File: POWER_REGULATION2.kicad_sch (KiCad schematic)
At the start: 73 parts, among them Q8 FDV301N, U19 NL17SZ17XV5T2G, U21 NC7WZ07P6X, U22 TPS65400RGZT, U40 TPS22918DBVR, U9 SIP32510DT-T1-GE3

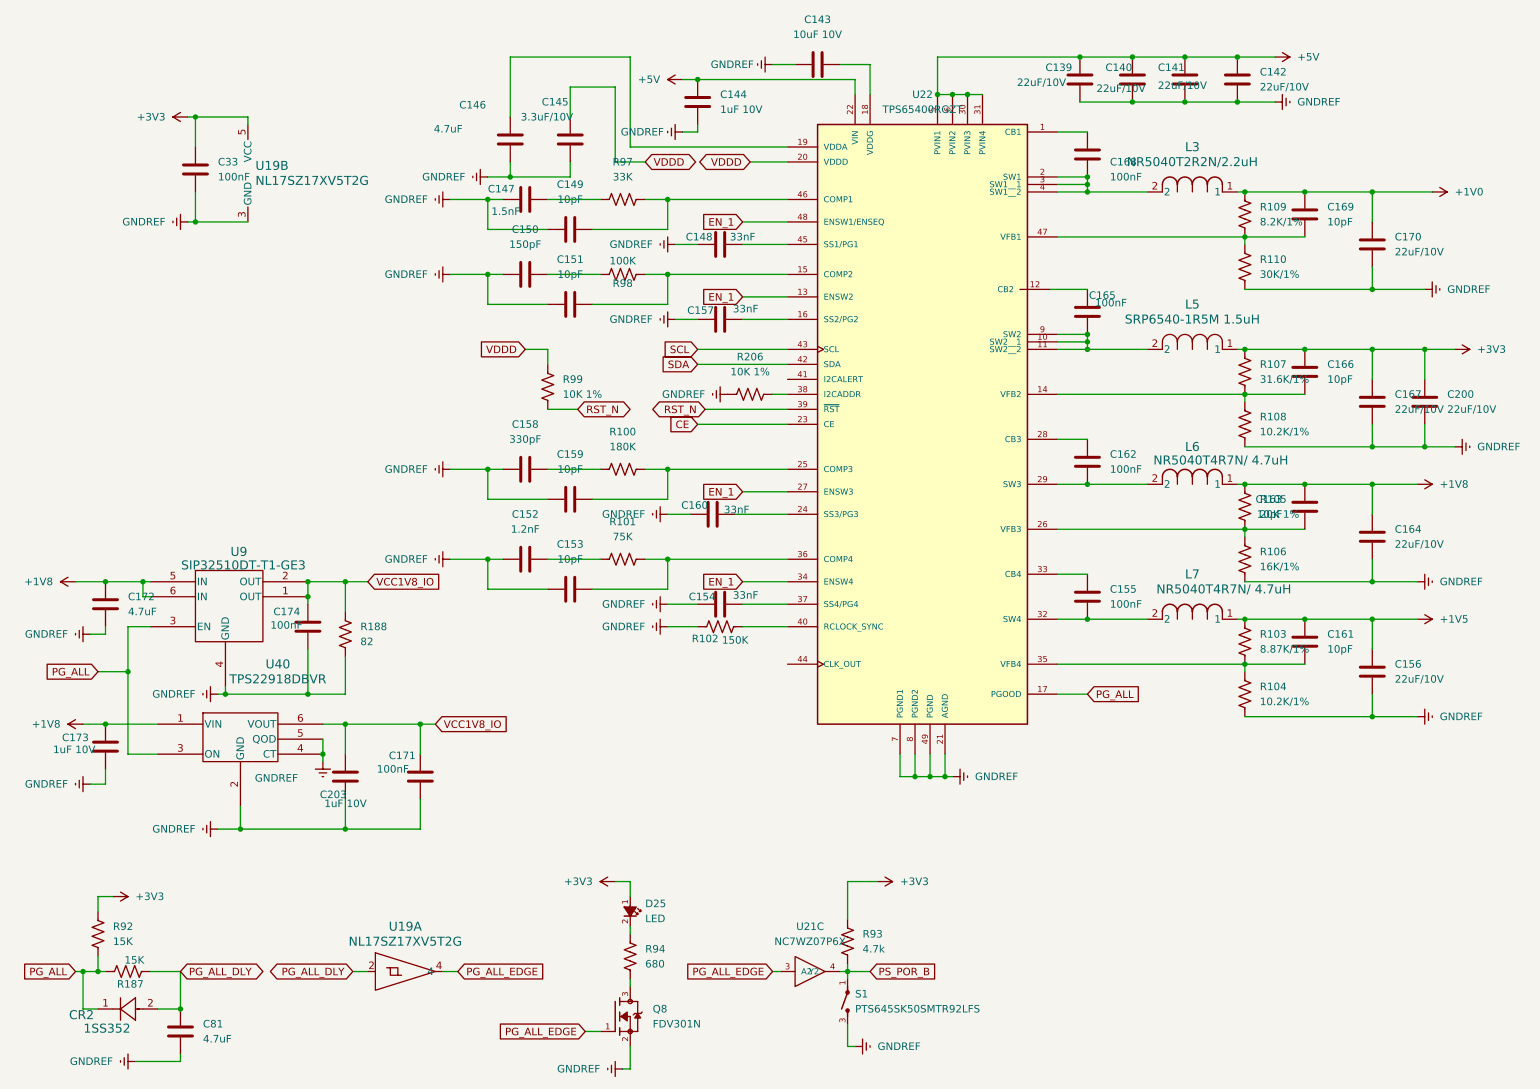
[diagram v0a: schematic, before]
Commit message: post -production rework
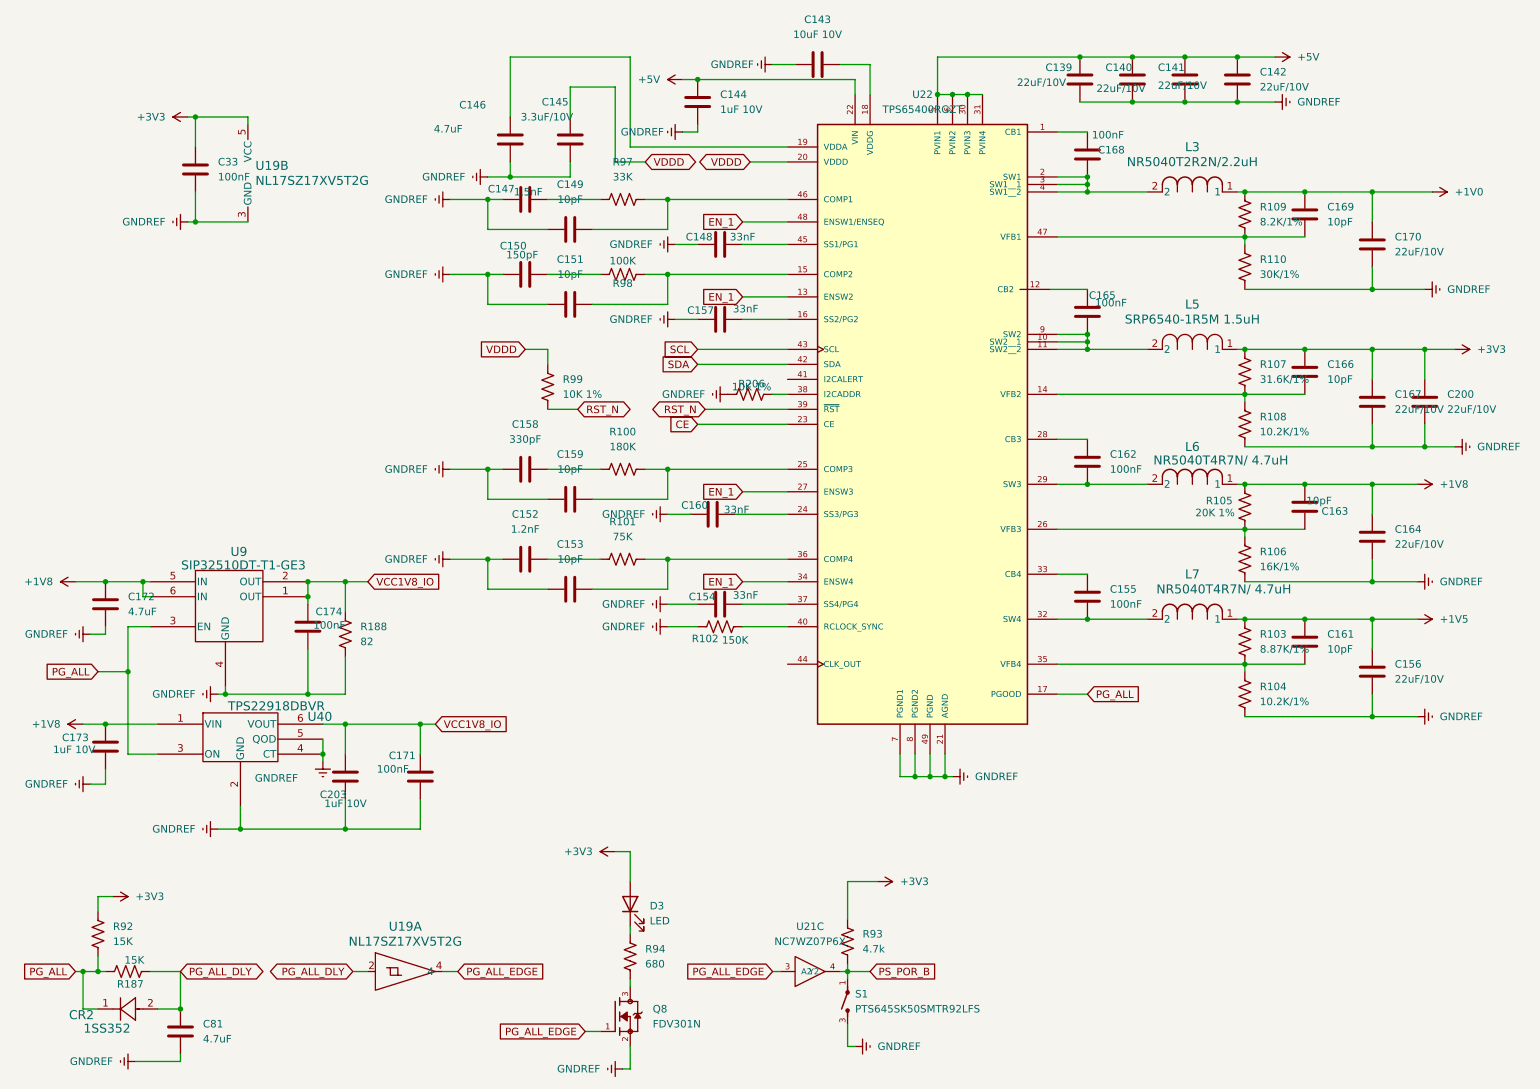
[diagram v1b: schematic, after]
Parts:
- removed D25: LED, footprints:LED_0402_1005Metric, symbol Aquiot:LED
- added D3: LED, footprints:LED_0402_1005Metric, symbol Device:LED
- C152: LCSC PN C18213195 -> C913747
- C161, C163, C166, C169, C171, C173, C200, C203, U40: now left out of the parts list
- R94: LCSC PN C307010 -> C158391
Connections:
- net +3V3: now also D3.2 (A)
- net at R94.1: now also D3.1 (K)
